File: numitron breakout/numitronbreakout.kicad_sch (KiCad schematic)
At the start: 13 parts, among them J1 Conn_01x06, U1 HV5812WG-G, U2 LM317_TO-220, U3 LM317_TO-220, U4 IV-12, U5 IV-12

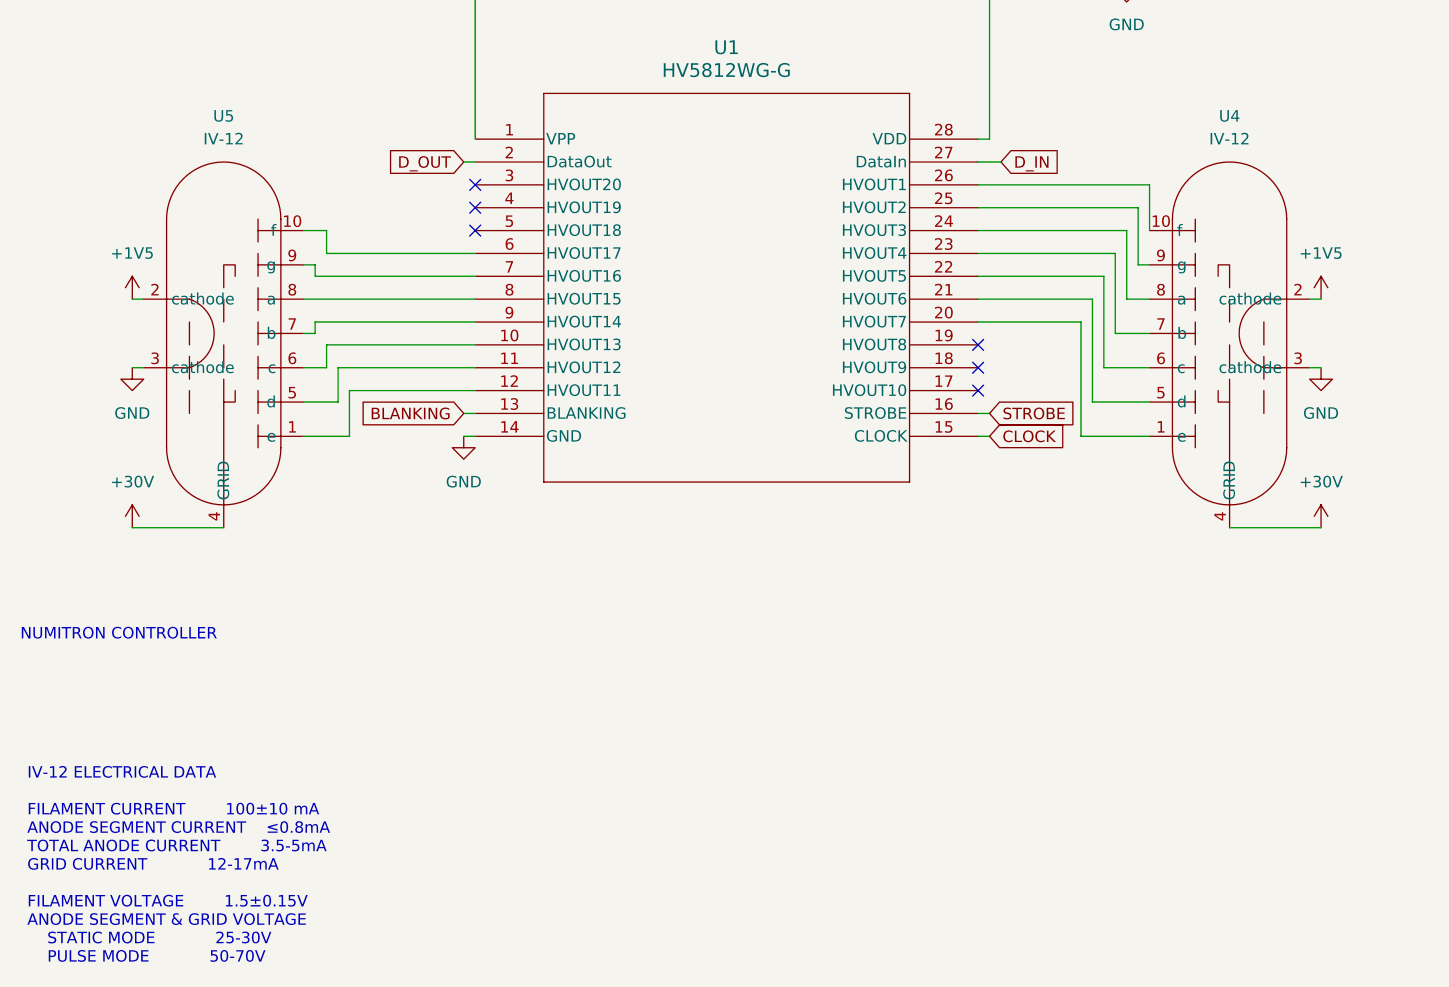
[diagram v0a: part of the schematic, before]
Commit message: code attempt, small layout updates
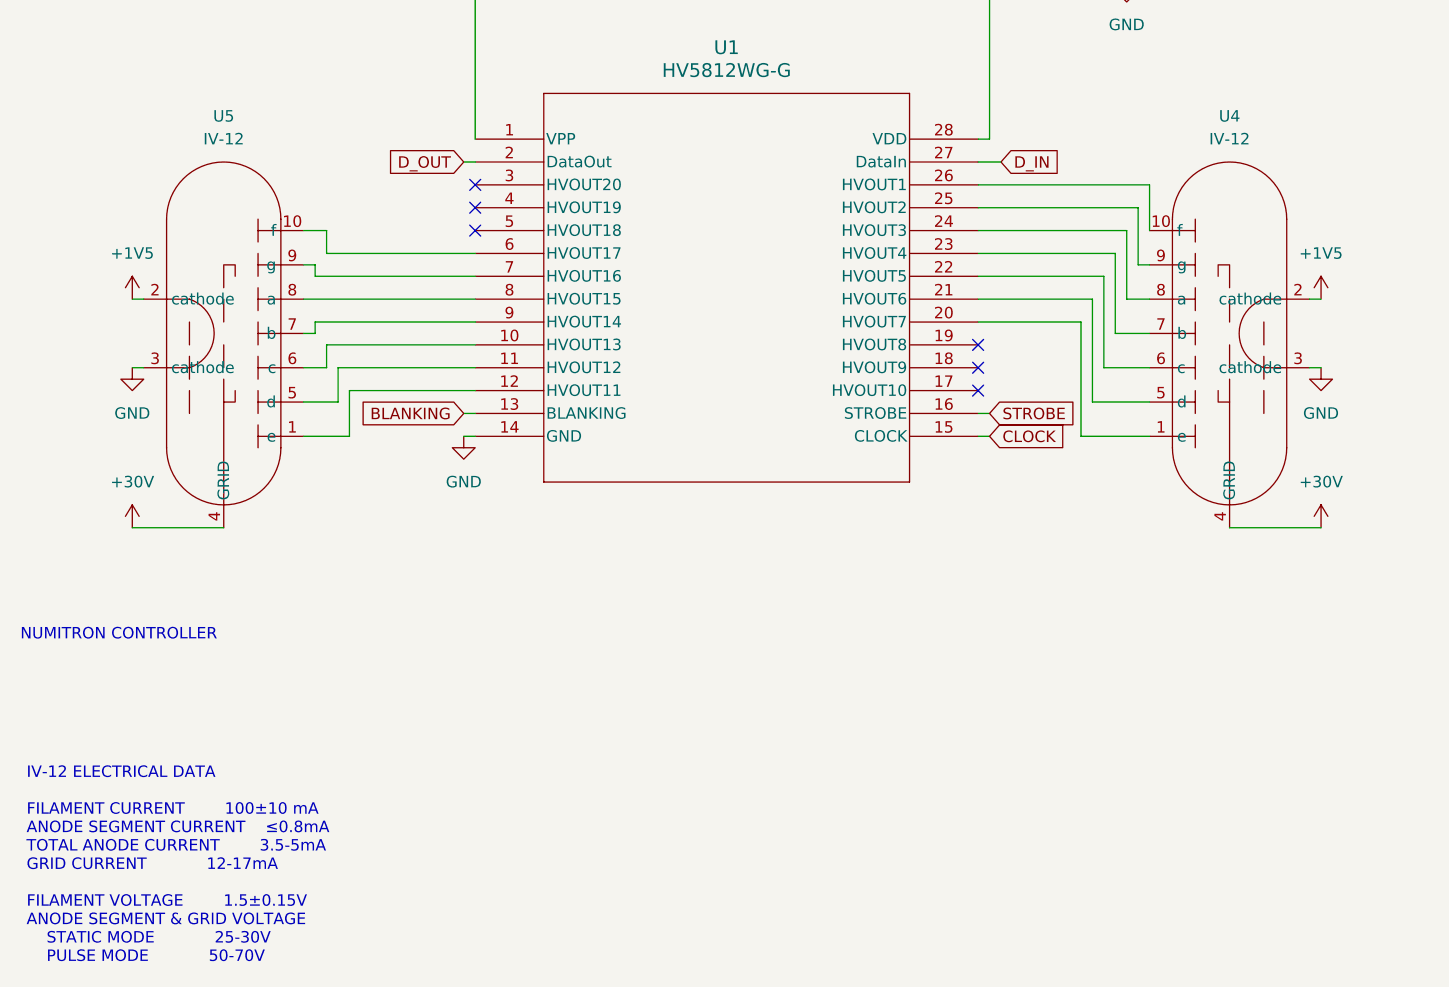
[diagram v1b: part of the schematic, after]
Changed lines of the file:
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@@
 (kicad_sch
-	(version 20231120)
+	(version 20250114)
 	(generator "eeschema")
-	(generator_version "8.0")
+	(generator_version "9.0")
 	(paper "USLetter")
 	(title_block
@@
 		(company "AL LEVINE")
 	)
+	(text "INPUT PINS"
+		(exclude_from_sim no)
+		(at 12.7 63.5 0)
+		(effects
+			(font
+				(size 1.27 1.27)
+			)
+			(justify left bottom)
+		)
+	)
+	(text "DC-DC REGULATOR 12V TO 1.5V"
+		(exclude_from_sim no)
+		(at 63.5 63.754 0)
+		(effects
+			(font
+				(size 1.27 1.27)
+			)
+			(justify left bottom)
+		)
+	)
+	(text "DC-DC REGULATOR 12V TO 32V"
+		(exclude_from_sim no)
+		(at 178.054 63.5 0)
+		(effects
+			(font
+				(size 1.27 1.27)
+			)
+			(justify left bottom)
+		)
+	)
+	(text "DC-DC REGULATOR 12V TO 5V"
+		(exclude_from_sim no)
+		(at 127 63.754 0)
+		(effects
+			(font
+				(size 1.27 1.27)
+			)
+			(justify left bottom)
+		)
+	)
+	(text "NUMITRON CONTROLLER"
+		(exclude_from_sim no)
+		(at 12.954 165.1 0)
+		(effects
+			(font
+				(size 1.27 1.27)
+			)
+			(justify left bottom)
+		)
+	)
+	(text_box "IV-12 ELECTRICAL DATA\n\nFILAMENT CURRENT		100±10 mA\nANODE SEGMENT CURRENT	≤0.8mA\nTOTAL ANODE CURRENT		3.5-5mA\nGRID CURRENT			12-17mA\n\nFILAMENT VOLTAGE		1.5±0.15V\nANODE SEGMENT & GRID VOLTAGE\n	STATIC MODE			25-30V\n	PULSE MODE			50-70V"
+		(exclude_from_sim no)
+		(at 12.7 177.8 0)
+		(size 50.8 25.4)
+		(margins 0.9524 0.9524 0.9524 0.9524)
+		(stroke
+			(width -0.0001)
+			(type default)
+		)
+		(fill
+			(type none)
+		)
+		(effects
+			(font
+				(size 1.27 1.27)
+			)
+			(justify left top)
+		)
+	)
 	(junction
 		(at 241.3 45.72)
@@
 		)
 	)
-	(text_box "IV-12 ELECTRICAL DATA\n\nFILAMENT CURRENT		100±10 mA\nANODE SEGMENT CURRENT	≤0.8mA\nTOTAL ANODE CURRENT		3.5-5mA\nGRID CURRENT			12-17mA\n\nFILAMENT VOLTAGE		1.5±0.15V\nANODE SEGMENT & GRID VOLTAGE\n	STATIC MODE			25-30V\n	PULSE MODE			50-70V"
-		(exclude_from_sim no)
-		(at 12.7 177.8 0)
-		(size 50.8 25.4)
-		(stroke
-			(width -0.0001)
-			(type default)
-		)
-		(fill
-			(type none)
-		)
-		(effects
-			(font
-				(size 1.27 1.27)
-			)
-			(justify left top)
-		)
-	)
-	(text "INPUT PINS"
-		(exclude_from_sim no)
-		(at 12.7 63.5 0)
-		(effects
-			(font
-				(size 1.27 1.27)
-			)
-			(justify left bottom)
-		)
-	)
-	(text "DC-DC REGULATOR 12V TO 1.5V"
-		(exclude_from_sim no)
-		(at 63.5 63.754 0)
-		(effects
-			(font
-				(size 1.27 1.27)
-			)
-			(justify left bottom)
-		)
-	)
-	(text "DC-DC REGULATOR 12V TO 32V"
-		(exclude_from_sim no)
-		(at 178.054 63.5 0)
-		(effects
-			(font
-				(size 1.27 1.27)
-			)
-			(justify left bottom)
-		)
-	)
-	(text "DC-DC REGULATOR 12V TO 5V"
-		(exclude_from_sim no)
-		(at 127 63.754 0)
-		(effects
-			(font
-				(size 1.27 1.27)
-			)
-			(justify left bottom)
-		)
-	)
-	(text "NUMITRON CONTROLLER"
-		(exclude_from_sim no)
-		(at 12.954 165.1 0)
-		(effects
-			(font
-				(size 1.27 1.27)
-			)
-			(justify left bottom)
-		)
-	)
 	(global_label "D_OUT"
 		(shape input)
@@
 		)
 	)
+	(embedded_fonts no)
 )
